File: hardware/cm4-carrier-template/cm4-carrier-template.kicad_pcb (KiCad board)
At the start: 4 copper layers, 90 x 90 mm, 26 parts, among them J1 USB_C_Receptacle_USB2.0, J2 Micro_SD_Card, J3 Abracon_ARJ-139, U1 TPD2EUSB30, U2 TPD2EUSB30, U3 TPD2EUSB30, U4 TPD2EUSB30, U5 Compute_Module_4_Functional, U6 Expansion_PoE

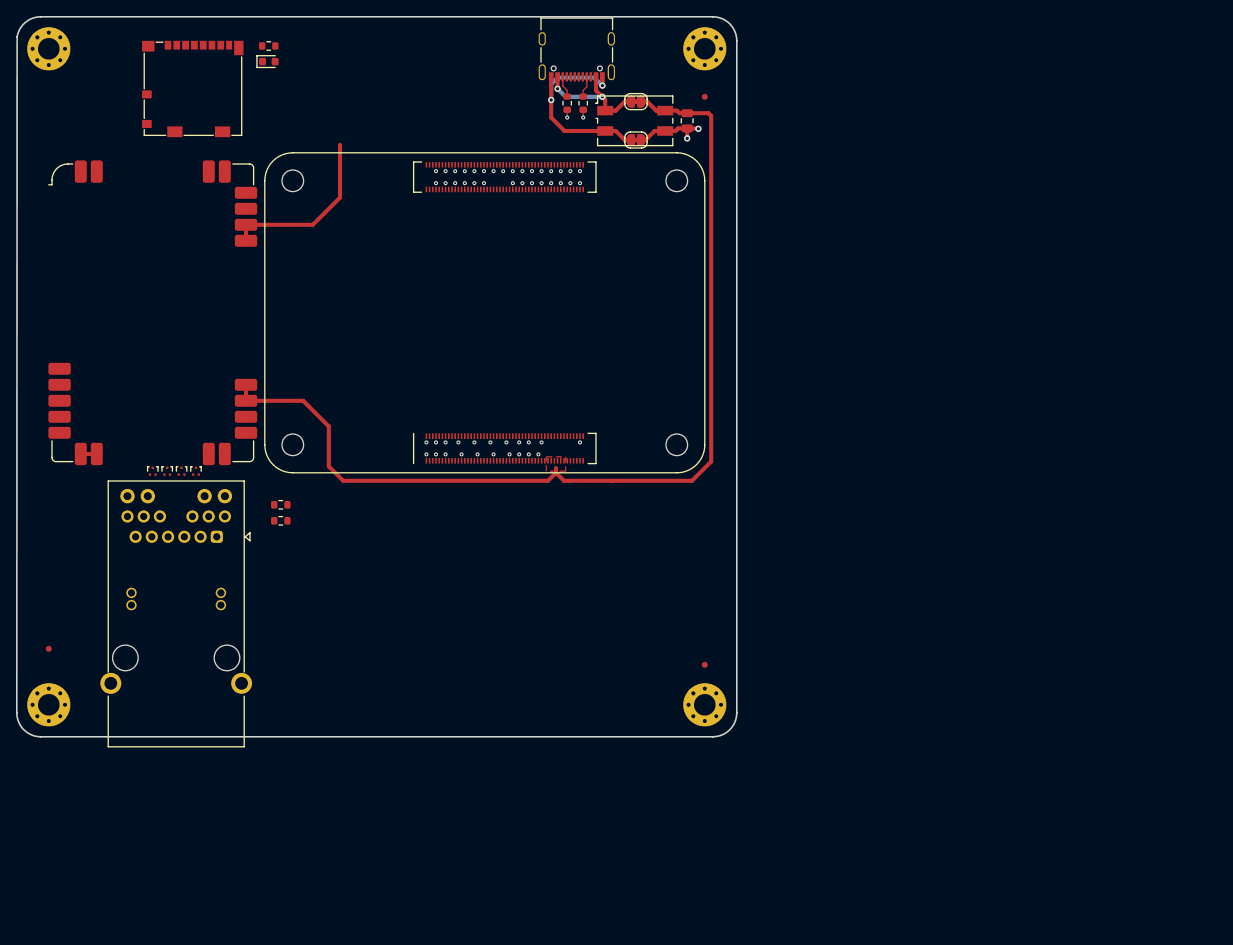
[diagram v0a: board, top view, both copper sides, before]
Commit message: Pre-stream commit.
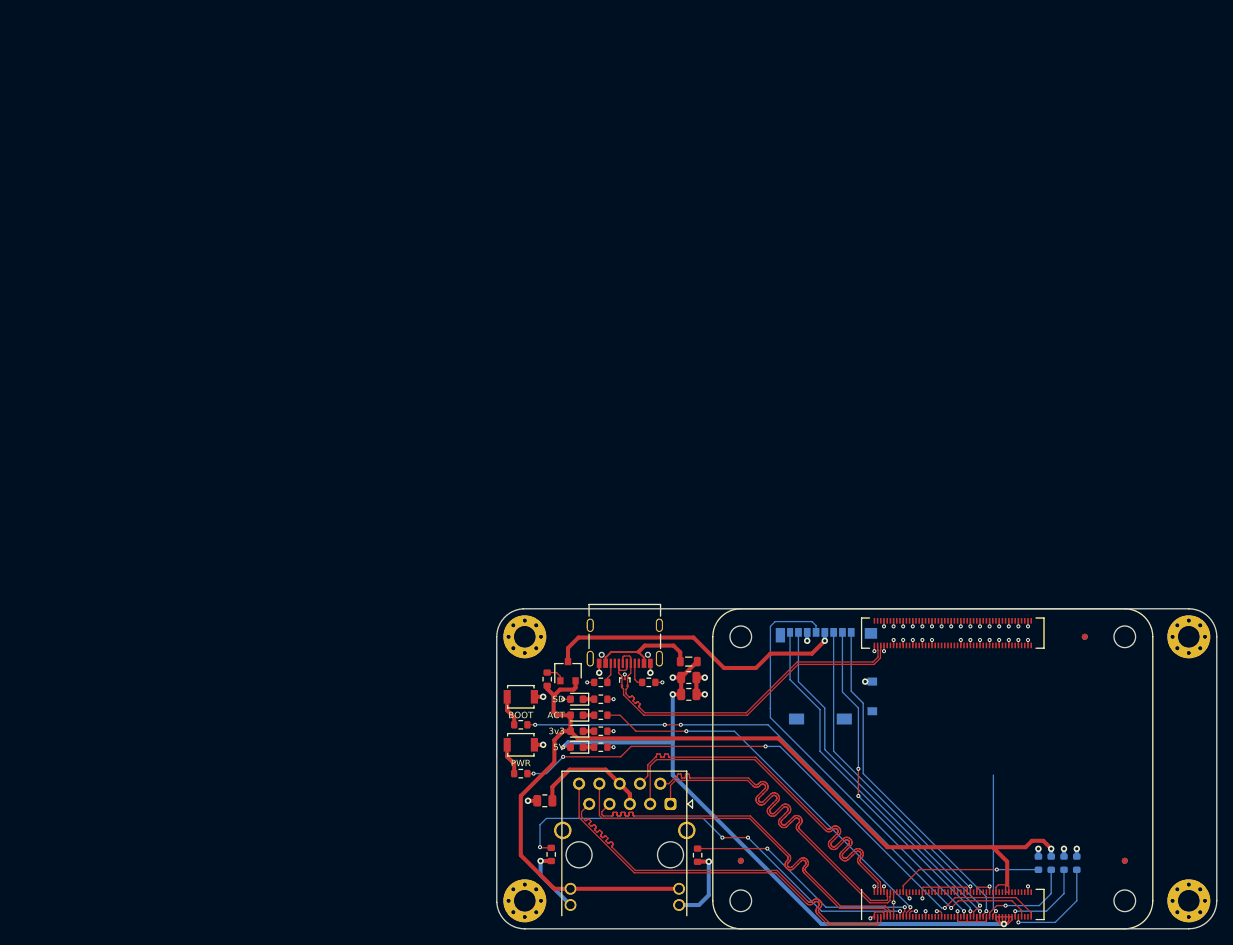
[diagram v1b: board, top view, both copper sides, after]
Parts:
- removed JP1: USB_VBUS, Jumper:SolderJumper-2_P1.3mm_Bridged_RoundedPad1.0x1.5mm
- removed JP2: USB_GND, Jumper:SolderJumper-2_P1.3mm_Bridged_RoundedPad1.0x1.5mm
- removed L1: DNP, Inductor_SMD:L_CommonMode_Wuerth_WE-SL2
- removed U1, U2, U3, U4: TPD2EUSB30, Package_TO_SOT_SMD:Texas_DRT-3
- added C2: 22u, Capacitor_SMD:C_0805_2012Metric, F.Cu at (104.0, 102.6)
- added C3: 100n, Capacitor_SMD:C_0805_2012Metric, F.Cu at (86.0, 118.0)
- added D2: RPi 3v3, LED_SMD:LED_0603_1608Metric, F.Cu at (90.0, 109.3)
- added D3: Activity LED, LED_SMD:LED_0603_1608Metric, F.Cu at (90.0, 107.3)
- added D4: SD ON, LED_SMD:LED_0603_1608Metric, F.Cu at (90.0, 105.3)
- added FB1: FB, Inductor_SMD:L_0805_2012Metric, F.Cu at (104.0, 100.6)
- added FID4: Fiducial, Fiducial:Fiducial_0.75mm_Mask1.5mm, B.Cu at (110.5, 125.5)
- added FID5: Fiducial, Fiducial:Fiducial_0.75mm_Mask1.5mm, B.Cu at (158.5, 125.5)
- added FID6: Fiducial, Fiducial:Fiducial_0.75mm_Mask1.5mm, B.Cu at (153.5, 97.5)
- added Q1: DMP2066LSN, Package_TO_SOT_SMD:SC-59, F.Cu at (88.9, 101.8)
- added R10: 220R, Resistor_SMD:R_0603_1608Metric, F.Cu at (93.0, 107.3)
- added R11: 220R, Resistor_SMD:R_0603_1608Metric, F.Cu at (83.0, 114.6)
- added R12: 220R, Resistor_SMD:R_0603_1608Metric, F.Cu at (93.0, 105.3)
- added R13: 0R, Resistor_SMD:R_0603_1608Metric, B.Cu at (150.9, 125.8)
- added R14: 0R, Resistor_SMD:R_0603_1608Metric, B.Cu at (152.5, 125.8)
- added R15: 0R, Resistor_SMD:R_0603_1608Metric, B.Cu at (147.7, 125.8)
- added R6: 330R, Resistor_SMD:R_0603_1608Metric, F.Cu at (93.0, 111.3)
- added R7: 220R, Resistor_SMD:R_0603_1608Metric, F.Cu at (93.0, 109.3)
- added R8: 220R, Resistor_SMD:R_0603_1608Metric, F.Cu at (86.3, 102.8)
- added R9: 220R, Resistor_SMD:R_0603_1608Metric, F.Cu at (83.0, 108.5)
- added SW1: BOOT, Button_Switch_SMD:SW_SPST_B3U-1000P, F.Cu at (83.0, 105.0)
- added SW2: GLOBAL_EN, Button_Switch_SMD:SW_SPST_B3U-1000P, F.Cu at (83.0, 111.0)
- D1: value SD ON -> USB Power; footprint Diode_SMD:D_0603_1608Metric -> LED_SMD:LED_0603_1608Metric
- J2: moved to B.Cu
- J3: value Abracon_ARJ-139 -> Abracon_ARJM11-502; footprint jkiv-library:RJ45_Abracon_ARJ136 -> jkiv-library:RJ45_Abracon_ARJM11
- R3, R4: value 100R -> 220R
- R5: value 100R -> DNP; moved to B.Cu
- U6: value Expansion_PoE -> TPD2EUSB30; footprint jkiv-library:expansion-poe-P2.0mm_SMD -> Package_TO_SOT_SMD:Texas_DRT-3
- moved R5 141.4 mm to (149.3, 125.8), turned to 90 degrees
- moved FID3 129.5 mm to (153.5, 97.5)
- moved H4 122.5 mm to (166.5, 130.5)
- moved FID2 109.0 mm to (158.5, 125.5)
- moved J2 108.0 mm to (121.2, 102.4), turned to 180 degrees
- moved H1 94.6 mm to (83.5, 97.5)
- moved D1 94.0 mm to (90.0, 111.3), turned to 180 degrees
- moved U5 79.9 mm to (137.0, 114.0)
- moved U6 74.9 mm to (96.0, 103.2)
- moved J1 73.5 mm to (96.0, 98.3)
- moved R1 72.9 mm to (99.0, 103.2), turned to 180 degrees
- moved R2 72.5 mm to (93.0, 103.2), turned to 0 degrees
- moved C1 71.7 mm to (104.0, 104.7), turned to 0 degrees
- moved R3 66.8 mm to (105.1, 124.8), turned to 90 degrees
- moved J3 65.8 mm to (101.7, 118.4)
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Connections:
- D1 pad 2: Net-(D1-Pad2) -> +5V
- J1 pad A1: /USB_GND -> GND
- J1 pad A12: /USB_GND -> GND
- J1 pad A6: Net-(J1-PadA6) -> /USB_D+
- J1 pad A7: Net-(J1-PadA7) -> /USB_D-
- J1 pad B1: /USB_GND -> GND
- J1 pad B12: /USB_GND -> GND
- J1 pad B6: Net-(J1-PadB6) -> /USB_D+
- J1 pad B7: Net-(J1-PadB7) -> /USB_D-
- J2 pad 4: +3V3 -> /SD_PWR
- J3 pad 1: Net-(J3-Pad1) -> /E0_TR0+
- J3 pad 10: /E0_TR0- -> /E0_TR3-
- J3 pad 11: /E0_TR0+ -> +3V3
- J3 pad 12: Net-(J3-Pad1) -> Net-(J3-Pad12)
- J3 pad 13: /PoE_TAP1 -> +3V3
- J3 pad 14: /PoE_TAP2 -> Net-(J3-Pad14)
- J3 pad 2: /E0_TR2- -> /E0_TR0-
- J3 pad 3: /E0_TR2+ -> /E0_TR1+
- J3 pad 4: /E0_TR1+ -> /E0_TR1-
- J3 pad 5: /E0_TR1- -> Net-(C3-Pad1)
- J3 pad 6: Net-(J3-Pad1) -> Net-(C3-Pad1)
- J3 pad 7: Net-(J3-Pad1) -> /E0_TR2+
- J3 pad 8: /E0_TR3+ -> /E0_TR2-
- J3 pad 9: /E0_TR3- -> /E0_TR3+
- J3 pad SH: GNDREF -> GND
- R3 pad 1: Net-(J3-Pad18) -> Net-(J3-Pad14)
- R4 pad 1: Net-(J3-Pad19) -> Net-(J3-Pad12)
- R5 pad 1: Net-(D1-Pad1) -> Net-(R5-Pad1)
- R5 pad 2: GND -> +3V3
- U5 pad 101: Net-(U5-Pad101) -> GND
- U5 pad 21: Net-(U5-Pad21) -> /PI_LED_nACT
- U5 pad 73: Net-(U5-Pad73) -> Net-(R5-Pad1)
- U5 pad 75: Net-(D1-Pad2) -> /SD_PWR_ON
- U5 pad 93: Net-(U5-Pad93) -> /PI_nRPI_BOOT
- U5 pad 99: Net-(U5-Pad99) -> /PI_GLOBAL_EN
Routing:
- net +3V3: track 0.00 -> 129.9 mm, vias 0 -> 1
- net /PI_GLOBAL_EN: track 0.00 -> 74.6 mm, vias 0 -> 4
- net /PI_nRPI_BOOT: track 0.00 -> 72.9 mm, vias 0 -> 4
- net GND: track 11.0 -> 71.8 mm, vias 55 -> 61
- net /~E0_LEDL: track 0.00 -> 55.1 mm, vias 0 -> 4
- net /SD_CLK: track 0.00 -> 53.4 mm, vias 0 -> 1
- net +5V: track 144.1 -> 90.9 mm, vias 0 -> 4
- net /E0_TR0-: track 0.00 -> 50.1 mm
- net /E0_TR0+: track 0.00 -> 50.1 mm
- net /E0_TR1-: track 0.00 -> 50.0 mm
- net /E0_TR1+: track 0.00 -> 50.0 mm
- net /E0_TR3+: track 0.00 -> 49.8 mm
- net /E0_TR3-: track 0.00 -> 49.8 mm
- net /PI_LED_nACT: track 0.00 -> 49.2 mm, vias 0 -> 2
- net /E0_TR2+: track 0.00 -> 49.0 mm
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- removed copper zone on F.Cu, net +5V
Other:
- board size 90 x 90 mm -> 90 x 40 mm
- board text added: "3v3"
- board text added: "5V"
- board text added: "ACT"
- board text added: "BOOT"
- board text added: "PWR"
- board text added: "SD"
- board text added: "~BT"
- board text added: "~EEPROM"
- board text added: "~SD"
- board text added: "~WiFi"
